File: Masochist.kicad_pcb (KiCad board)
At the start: 2 copper layers, 114.3 x 58.7 mm, 57 parts, among them J1 USB_C_Receptacle_USB2.0, SW1 SW_Push, U1 ATmega32U4-MU, U2 USBLC6-2SC6, Y1 16 MHz

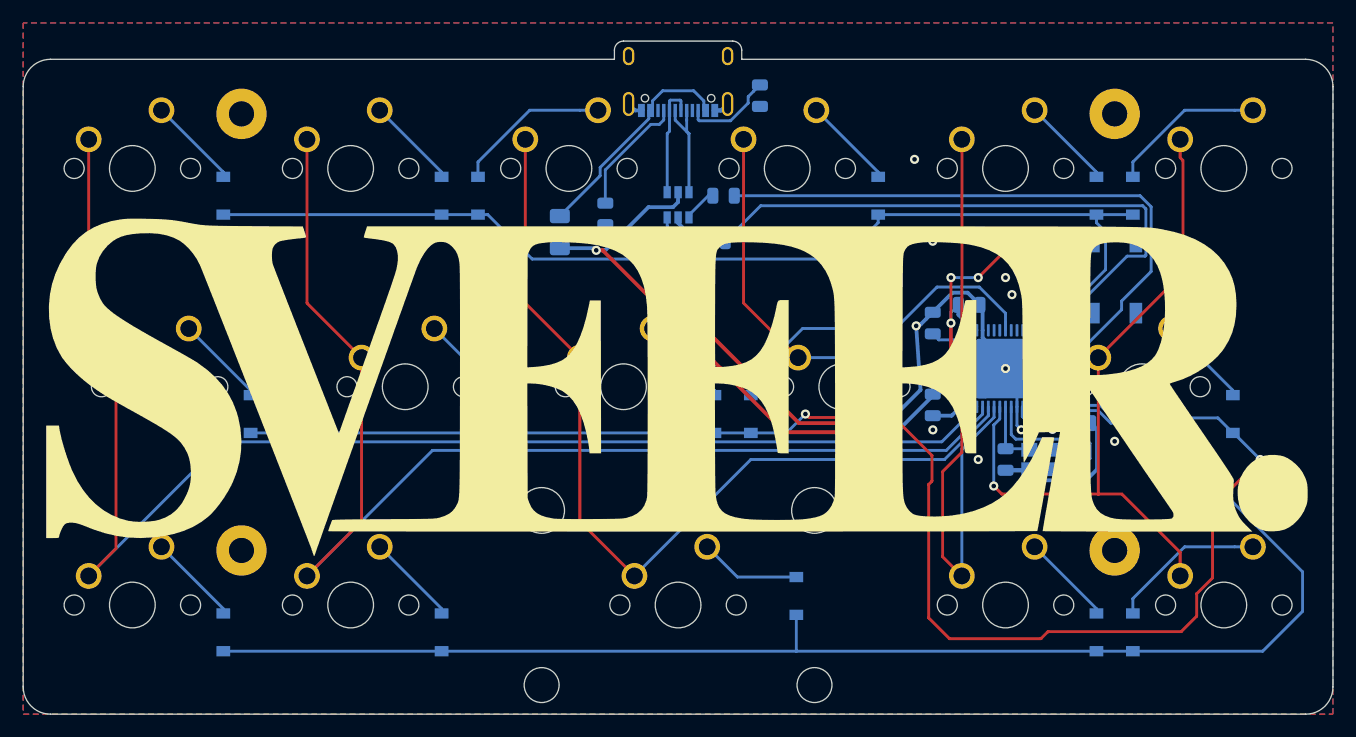
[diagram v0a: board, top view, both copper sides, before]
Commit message: add v1.1
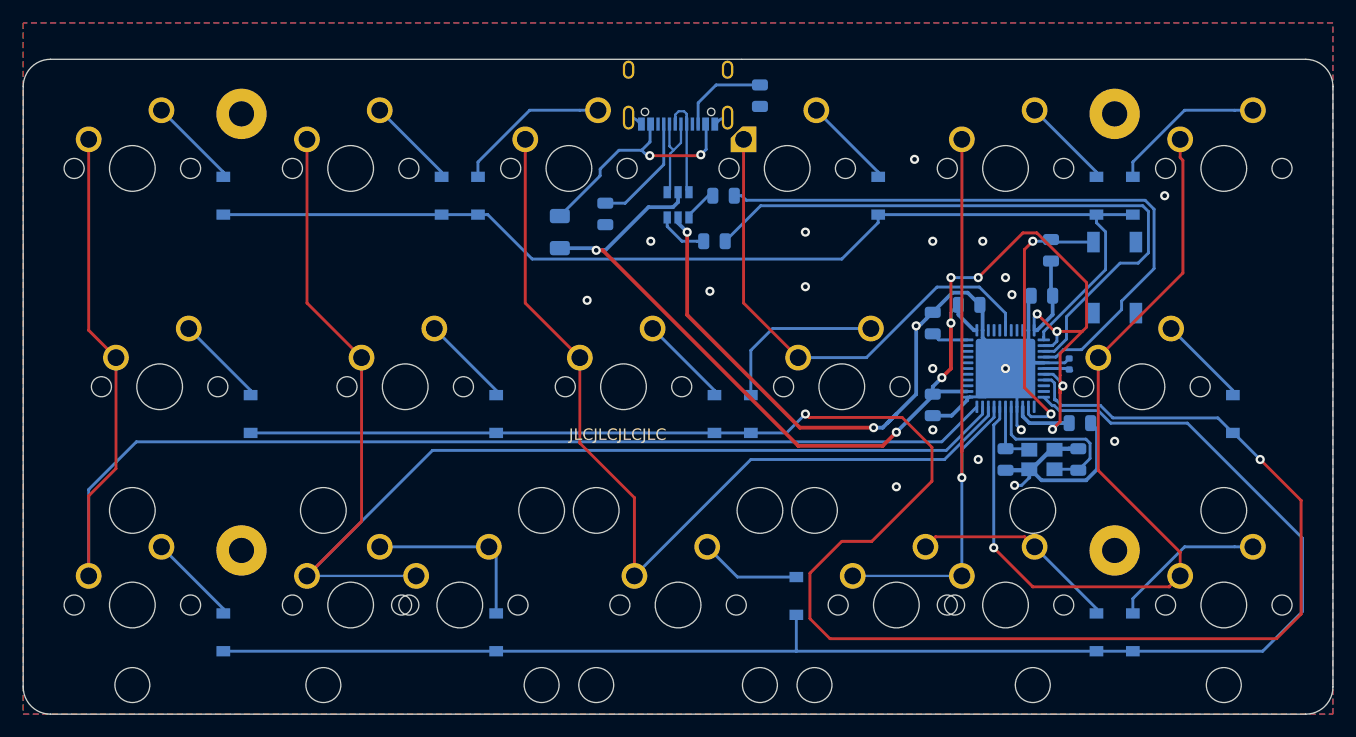
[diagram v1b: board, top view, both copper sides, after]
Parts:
- removed ?: , 
- removed the G*** at (83.3, 145.3)
- removed REF** (x3): MountingHole_2.2mm_M2_Pad, cftkb:MountingHole_2.2mm_M2_Pad
- added H1: MountingHole_Pad, MountingHole:MountingHole_2.2mm_M2_Pad, F.Cu at (45.2, 121.4)
- added H2: MountingHole_Pad, MountingHole:MountingHole_2.2mm_M2_Pad, F.Cu at (121.4, 121.4)
- added H3: MountingHole_Pad, MountingHole:MountingHole_2.2mm_M2_Pad, F.Cu at (45.2, 159.5)
- added H4: MountingHole_Pad, MountingHole:MountingHole_2.2mm_M2_Pad, F.Cu at (121.4, 159.5)
- added MX13: MX-NoLED, MX_Only:MXOnly-2U-ReversedStabilizers-NoLED, F.Cu at (102.4, 164.3)
- added MX6: MX-NoLED, MX_Only:MXOnly-2U-ReversedStabilizers-NoLED, F.Cu at (64.3, 164.3)
- added MX9: MX-NoLED, marbastlib-mx:STAB_MX_6u, F.Cu at (83.3, 164.3)
- C7: footprint Capacitor_SMD:C_0504_1310Metric -> Capacitor_SMD:C_0402_1005Metric
- moved D8 4.76 mm to (67.5, 166.7)
- moved J1 1.19 mm to (83.3, 118.7)
- moved C7 0.11 mm to (117.5, 143.3)
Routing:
- net Row1: track 139.7 -> 164.3 mm
- net Col5: track 62.0 -> 74.8 mm
- net Net-(D15-A): track 8.05 -> 18.3 mm
- net Col1: track 107.5 -> 117.0 mm
- net Net-(D8-A): track 8.05 -> 16.0 mm
- net Col0: track 123.7 -> 128.1 mm
- net Net-(U1-UCAP): track 2.40 -> 6.38 mm
- net D_BUS+: track 9.75 -> 12.0 mm
- net GND: track 104.7 -> 106.7 mm, vias 15 -> 22
- net D_BUS-: track 9.94 -> 8.12 mm
- net Row2: track 131.2 -> 132.9 mm
- net Net-(D13-A): track 13.6 -> 15.2 mm
- net +5V: track 123.5 -> 124.5 mm
- net Net-(J1-CC1): track 10.6 -> 9.65 mm
- net Col4: track 55.4 -> 55.9 mm, vias 0 -> 1
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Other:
- board size 114.3 x 58.7 mm -> 114.3 x 57.2 mm
- board text added: "JLCJLCJLCJLC"
- board text added: "Version 1.1"
